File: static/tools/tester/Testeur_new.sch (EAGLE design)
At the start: 30 parts, among them IC1 MEGA8-P

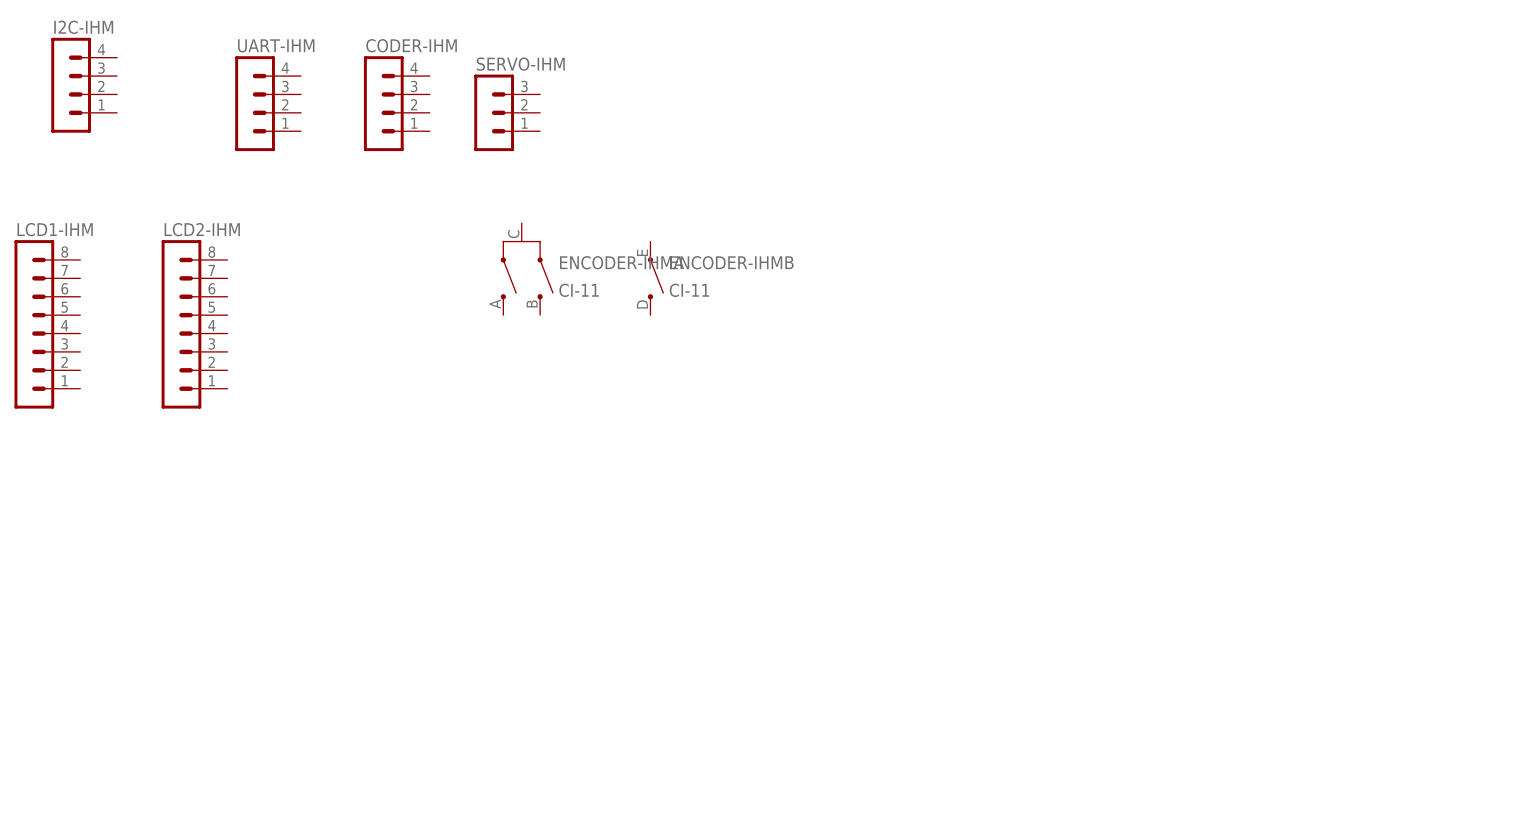
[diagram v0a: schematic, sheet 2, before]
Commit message: [tester] modify to V2 Alpha.
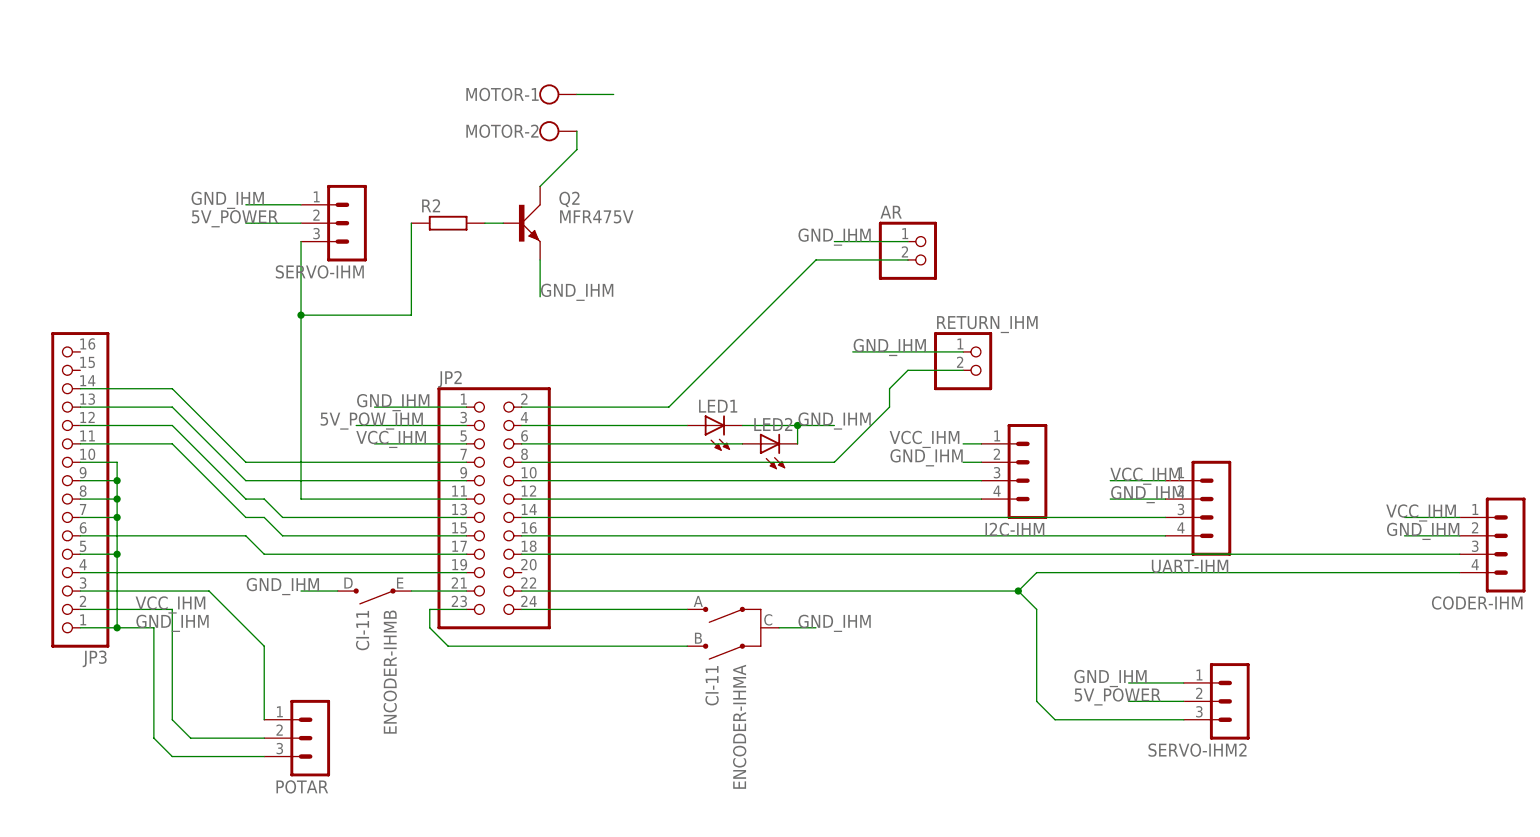
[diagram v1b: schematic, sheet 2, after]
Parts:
- removed CODER-MOTOR, I²C, SV1: (no value), con-lstb:MA04-1
- removed ENCODER-SELECT, LCD-GND: (no value), con-lstb:MA05-1
- removed LCD-CONTRASTE, POTAR-CONTRASTE, RETURN, SERVO/PWM: (no value), con-lstb:MA03-1
- removed LCD-DATA: (no value), con-lstb:MA06-1
- removed LCD1-IHM, LCD2-IHM: (no value), con-lstb:MA08-1
- added AR, RETURN_IHM: (no value), pinhead:PINHD-1X2
- added C1-REGULATOR1, C2-REGULATOR1: (no value), capacitor-wima:C5/5
- added IC3: (no value), v-reg:78XXS
- added JP1, JP2: (no value), pinhead:PINHD-2X12
- added JP3: (no value), pinhead:PINHD-1X16
- added MOTOR, X1: (no value), con-wago-500:W237-102
- added POTAR, SERVO-IHM2: (no value), con-lstb:MA03-1
- added Q2: MFR475V, transistor-power:MFR475V
- added R2: (no value), resistor:R-EU_0204/7
- ALIM: device con-lstb:MA03-1 -> pinhead:PINHD-1X2
- LED1, LED2: device led:LED3MM -> led:LED5MM
- R1: device rcl:R-EU_0204/5 -> rcl:R-EU_0204/7
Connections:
- net N$25 renamed LED1
- net N$26 renamed LED2
- removed net N$5: CODER-MOTOR.2, IC1.PD3(INT1)
- new net 5V_POWER: C2-REGULATOR1.1, IC3.OUT, SERVO-IHM.2, SERVO-IHM2.2
- new net 5V_POW_IHM: JP2.3
- new net ALIM_EXT: C1-REGULATOR1.1, IC3.IN, MOTOR-1.KL, X1-1.KL
- new net ENCODER1: IC1.PD4(XCK/T0), JP1.24
- new net ENCODER2: IC1.PD5(T1), JP1.23
- new net GND_IHM: AR.1, C1-REGULATOR1.2, C2-REGULATOR1.2, CODER-IHM.2, ENCODER-IHMA.C, ENCODER-IHMB.D, I2C-IHM.2, IC3.GND, JP2.1, JP3.1, JP3.10, JP3.5, JP3.7, JP3.8, JP3.9, LED1.C, LED2.C, POTAR.3, Q2.E, RETURN_IHM.1, SERVO-IHM.1, SERVO-IHM2.1, UART-IHM.2, X1-2.KL
- new net INT_ODO1: IC1.PD2(INT0), JP1.18
- new net LCD1: IC1.PD7(AIN1), JP1.19
- new net LCD2: IC1.PB0(ICP), JP1.17
- new net LCD3: IC1.PB1(OC1A), JP1.15
- new net LCD5: IC1.PB4(MISO), JP1.9
- new net LCD6: IC1.PB5(SCK), JP1.7
- new net N$25: JP2.19, JP3.4
- new net N$26: JP2.17, JP3.6
- new net N$34: JP2.7, JP3.14
- new net N$35: JP2.11, R2.1, SERVO-IHM.3
- new net N$36: JP2.8, RETURN_IHM.2
- new net N$37: AR.2, JP2.2
- new net N$39: JP3.3, POTAR.1
- new net N$40: MOTOR-2.KL, Q2.C
- new net RETURN: IC1.PC3(ADC3), JP1.8
- new net RX: IC1.PD0(RXD), JP1.14
- new net SCL: IC1.PC5(ADC5/SCL), JP1.12
- new net SDA: IC1.PC4(ADC4/SDA), JP1.10
- new net SELECT: IC1.PD6(AIN0), JP1.21
- new net SENS_ODO+SERVO2: IC1.PD3(INT1), JP1.22
- new net SERVO/PWM: IC1.PB3(MOSI/OC2), JP1.11
- new net TX: IC1.PD1(TXD), JP1.16
- new net VCC_IHM: CODER-IHM.1, I2C-IHM.1, JP2.5, JP3.2, POTAR.2, UART-IHM.1
- net GND: now also JP1.1; no longer CODER-MOTOR.4, ENCODER-SELECT.4, ENCODER-SELECT.5, I²C.2, LCD-CONTRASTE.3, LCD-GND.1, LCD-GND.2, LCD-GND.3, LCD-GND.4, LCD-GND.5, LED1.C, LED2.C, POTAR-CONTRASTE.3, RETURN.3, SERVO/PWM.3, SV1.3
- net N$10: now also I2C-IHM.3, JP2.10; no longer IC1.PB0(ICP), LCD-DATA.2
- net N$11: now also I2C-IHM.4, JP2.12; no longer IC1.PB3(MOSI/OC2), SERVO/PWM.1
- net N$12: now also JP2.4, LED1.A; no longer IC1.PB5(SCK), LCD-DATA.6
- net N$13: now also JP2.6, LED2.A; no longer IC1.PD7(AIN1), LCD-DATA.1
- net N$14: now also JP2.14, UART-IHM.3; no longer IC1.PB1(OC1A), LCD-DATA.3
- net N$15: now also JP2.16, UART-IHM.4; no longer IC1.PB2(SS/OC1B), LCD-DATA.4
- net N$16: now also CODER-IHM.3, JP2.18; no longer IC1.PB4(MISO), LCD-DATA.5
- net N$17: now also CODER-IHM.4, JP2.22, SERVO-IHM2.3; no longer CODER-MOTOR.1, IC1.PD2(INT0)
- net N$18: now also ENCODER-IHMA.A, JP2.24; no longer LED2.A, R3.2
- net N$21: now also ENCODER-IHMA.B, JP2.23; no longer IC1.PD0(RXD), SV1.1
- net N$22: now also ENCODER-IHMB.E, JP2.21; no longer IC1.PD1(TXD), SV1.2
- net N$27: now also JP2.15, JP3.11; no longer IC1.PC3(ADC3), RETURN.1
- net N$28: now also JP1.4; no longer LED1.A
- net N$29: now also JP2.13, JP3.12; no longer IC1.PC4(ADC4/SDA), I²C.3
- net N$3: now also IC1.PC0(ADC0), JP1.2; no longer LCD-CONTRASTE.1, POTAR-CONTRASTE.1
- net N$30: now also JP2.9, JP3.13; no longer IC1.PC5(ADC5/SCL), I²C.4
- net N$6: now also ALIM.2; no longer ALIM.3
- net N$7: now also JP1.6, R3.2; no longer ENCODER-SELECT.1, IC1.PD4(XCK/T0)
- net N$8: now also Q2.B, R2.2; no longer ENCODER-SELECT.2, IC1.PD5(T1)
- net N$9: now also IC1.PB2(SS/OC1B), JP1.13; no longer ENCODER-SELECT.3, IC1.PD6(AIN0)
- net VCC: now also JP1.5; no longer CODER-MOTOR.3, I²C.1, LCD-CONTRASTE.2, POTAR-CONTRASTE.2, SERVO/PWM.2, SV1.4
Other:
- moved on the sheet: CODER-IHM, ENCODER-IHMA, ENCODER-IHMB, I2C-IHM, R3, R4, SERVO-IHM, UART-IHM
